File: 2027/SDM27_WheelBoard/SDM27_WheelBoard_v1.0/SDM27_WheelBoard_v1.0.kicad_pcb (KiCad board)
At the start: 2 copper layers, 52 parts, among them IC1 NCP187AMT330TAG, IC8 TCAN3403DRBRQ1, IC9 MAX9924UAUB+, J1 5V, J2 GND, J3 GND, U1 ESP32-C5, U2 USBLC6-2SC6, Y1 Crystal_GND24

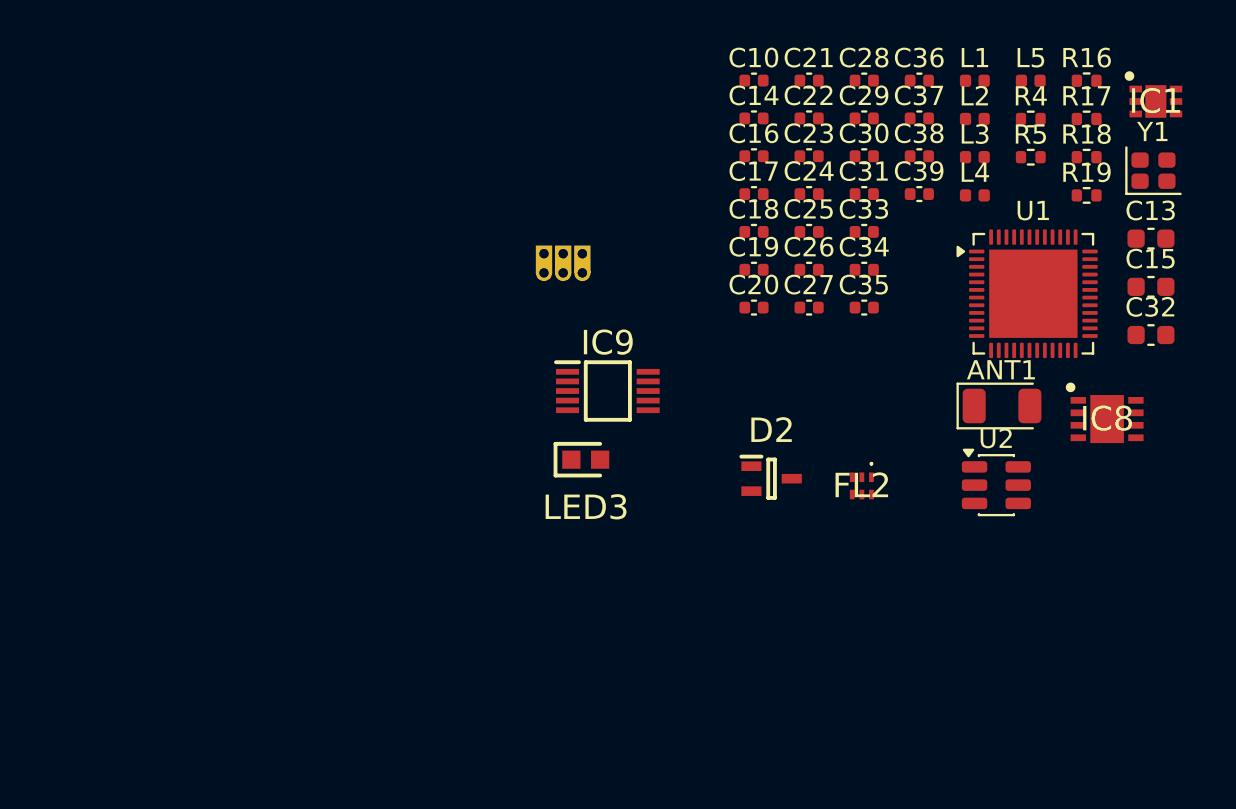
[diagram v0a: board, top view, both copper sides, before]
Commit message: more edits, board still very WIP. need to add USB
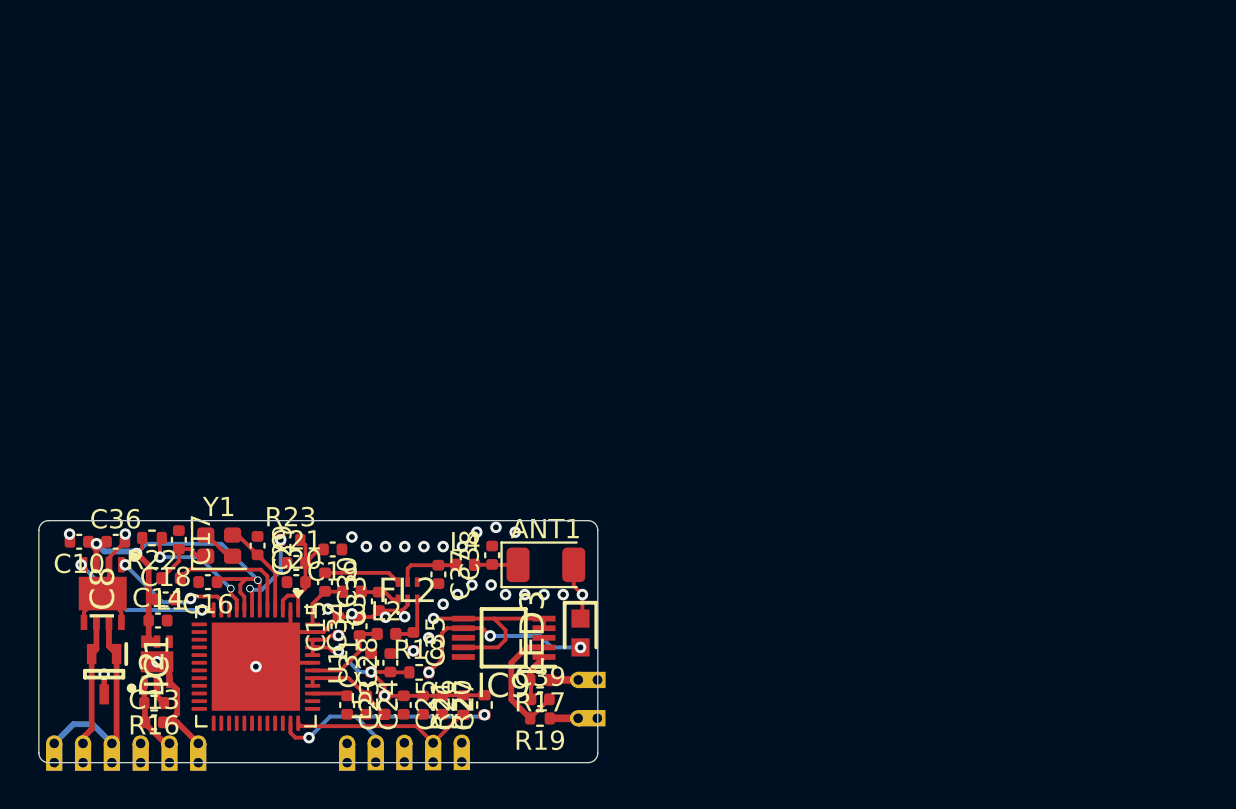
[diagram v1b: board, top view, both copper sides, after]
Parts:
- removed C22: 0.1uF, Capacitor_SMD:C_0402_1005Metric
- removed C32: 0.1uF, Capacitor_SMD:C_0603_1608Metric
- removed R4, R5: 27, Resistor_SMD:R_0402_1005Metric
- removed U2: USBLC6-2SC6, Package_TO_SOT_SMD:SOT-23-6
- added J10: WS+, SDM:DoublePin1.00mm, F.Cu at (117.8, 100.7)
- added J11: WS-, SDM:DoublePin1.00mm, F.Cu at (117.8, 102.7)
- added J12: CAN+, SDM:DoublePin1.00mm, F.Cu at (92.5, 105.0)
- added J13: CAN-, SDM:DoublePin1.00mm, F.Cu at (91.0, 105.0)
- added J4: CAN-, SDM:DoublePin1.00mm, F.Cu at (94.0, 105.0)
- added J5: 5V, SDM:DoublePin1.00mm, F.Cu at (110.7, 105.0)
- added J6: GND, SDM:DoublePin1.00mm, F.Cu at (107.7, 105.0)
- added J7: SDA, SDM:DoublePin1.00mm, F.Cu at (109.2, 105.0)
- added J8: SCL, SDM:DoublePin1.00mm, F.Cu at (106.2, 105.0)
- added J9: GND, SDM:DoublePin1.00mm, F.Cu at (104.8, 105.0)
- added R20: 4.7k, Resistor_SMD:R_0402_1005Metric, F.Cu at (111.9, 102.0)
- added R21: 4.7k, Resistor_SMD:R_0402_1005Metric, F.Cu at (110.8, 102.0)
- added R22: 10k, Resistor_SMD:R_0402_1005Metric, F.Cu at (94.6, 93.3)
- added R23: 10k, Resistor_SMD:R_0402_1005Metric, F.Cu at (101.8, 93.4)
- C13, C15: footprint Capacitor_SMD:C_0603_1608Metric -> Capacitor_SMD:C_0402_1005Metric
- J3: value GND -> CAN+
- moved IC1 59.6 mm to (94.8, 99.8), turned to 90 degrees
- moved R16 58.4 mm to (94.7, 101.9), turned to 180 degrees
- moved C13 57.7 mm to (94.7, 102.9)
- moved IC8 53.1 mm to (92.0, 96.2), turned to -90 degrees
- moved Y1 52.4 mm to (98.1, 93.7)
- moved L1 49.2 mm to (95.6, 95.4), turned to 180 degrees
- moved C36 48.2 mm to (92.7, 93.5)
- moved L5 46.8 mm to (106.7, 102.0), turned to 90 degrees
- moved C15 45.8 mm to (104.3, 97.9), turned to 90 degrees
- moved U1 44.9 mm to (100.0, 100.0), turned to -90 degrees
- moved R18 43.9 mm to (108.5, 100.3)
- moved C10 42.6 mm to (90.8, 93.5), turned to 180 degrees
- moved R17 40.8 mm to (114.8, 100.7), turned to 180 degrees
- moved L2 40.7 mm to (106.8, 98.3)
- moved C14 40.6 mm to (94.9, 97.6)
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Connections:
- J1 pad 1: unconnected-(J1-Pin_1-Pad1) -> +5V
- J2 pad 1: unconnected-(J2-Pin_1-Pad1) -> GND
- J3 pad 1: unconnected-(J3-Pin_1-Pad1) -> /CAN+
- U1 pad 11: unconnected-(U1-MTMS/GPIO2/FSPIQ/ADC1_CH1-Pad11) -> /CAN_RTX
- U1 pad 12: unconnected-(U1-MTDI/GPIO3/ADC1_CH2-Pad12) -> /CAN_CTX
- U1 pad 22: /USB_D- -> unconnected-(U1-GPIO13/USB_D-/SDIO_DATA3-Pad22)
- U1 pad 23: /USB_D+ -> unconnected-(U1-GPIO14/USB_D+/SDIO_DATA2-Pad23)
- U1 pad 35: unconnected-(U1-GPIO25-Pad35) -> /SCL
- U1 pad 36: unconnected-(U1-GPIO26-Pad36) -> /SDA
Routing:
- net GND: track 0.00 -> 49.4 mm, vias 0 -> 31
- net +3.3V: track 0.00 -> 48.7 mm, vias 0 -> 7
- net /SCL: track 0.00 -> 13.0 mm, vias 0 -> 2
- net /CAN-: track 0.00 -> 11.4 mm
- net /CAN+: track 0.00 -> 10.4 mm
- net /HE_OUTPUT: track 0.00 -> 10.1 mm, vias 0 -> 3
- net /SDA: track 0.00 -> 9.63 mm
- net /CAN_CTX: track 0.00 -> 8.02 mm, vias 0 -> 2
- net Net-(IC9-IN-): track 0.00 -> 6.75 mm
- net /CAN_RTX: track 0.00 -> 6.72 mm, vias 0 -> 2
- net /GPIO0: track 0.00 -> 6.65 mm, vias 0 -> 2
- net Net-(U1-XTAL_P): track 0.00 -> 6.61 mm
- net Net-(U1-XTAL_N): track 0.00 -> 4.97 mm
- net Net-(U1-VDDA1): track 0.00 -> 4.94 mm
- net /CHIP_EN: track 0.00 -> 4.81 mm, vias 0 -> 2
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- added copper zone on In2.Cu, net +3.3V
- added copper zone on In1.Cu, net GND
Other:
- board outline added: 29.1 x 12.6 mm
- copper layers 2 -> 4
